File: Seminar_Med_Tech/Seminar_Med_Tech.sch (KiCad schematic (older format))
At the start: 25 parts

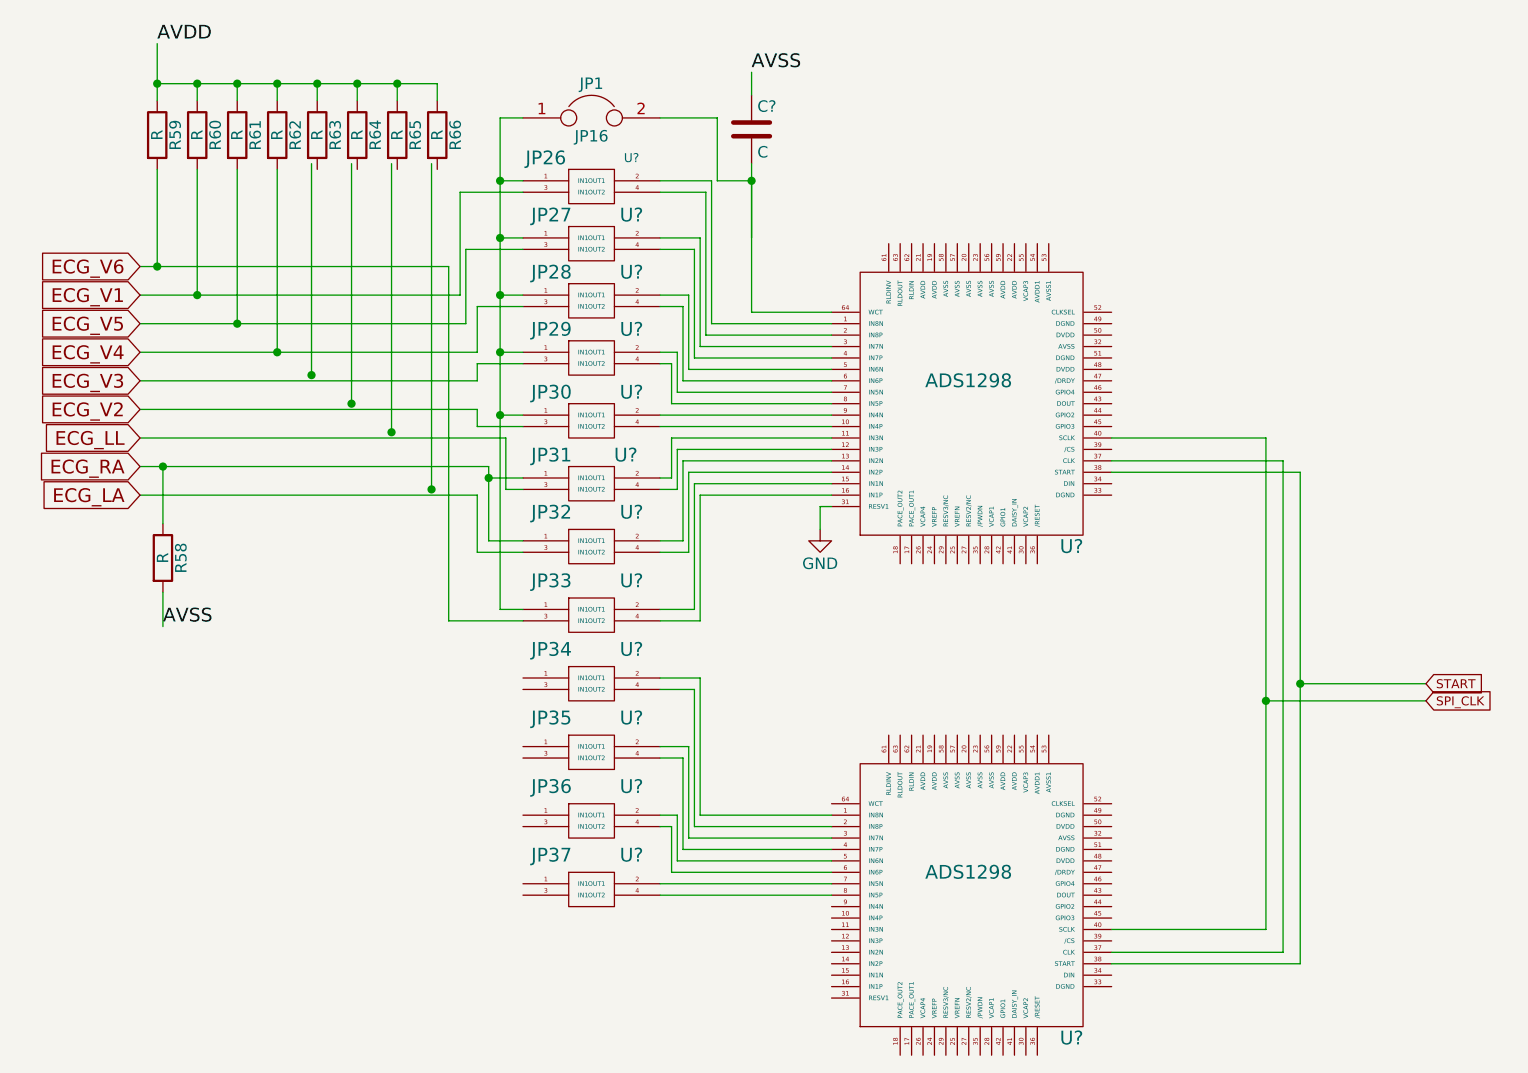
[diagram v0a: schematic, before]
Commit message: Tried to cascade the two chips
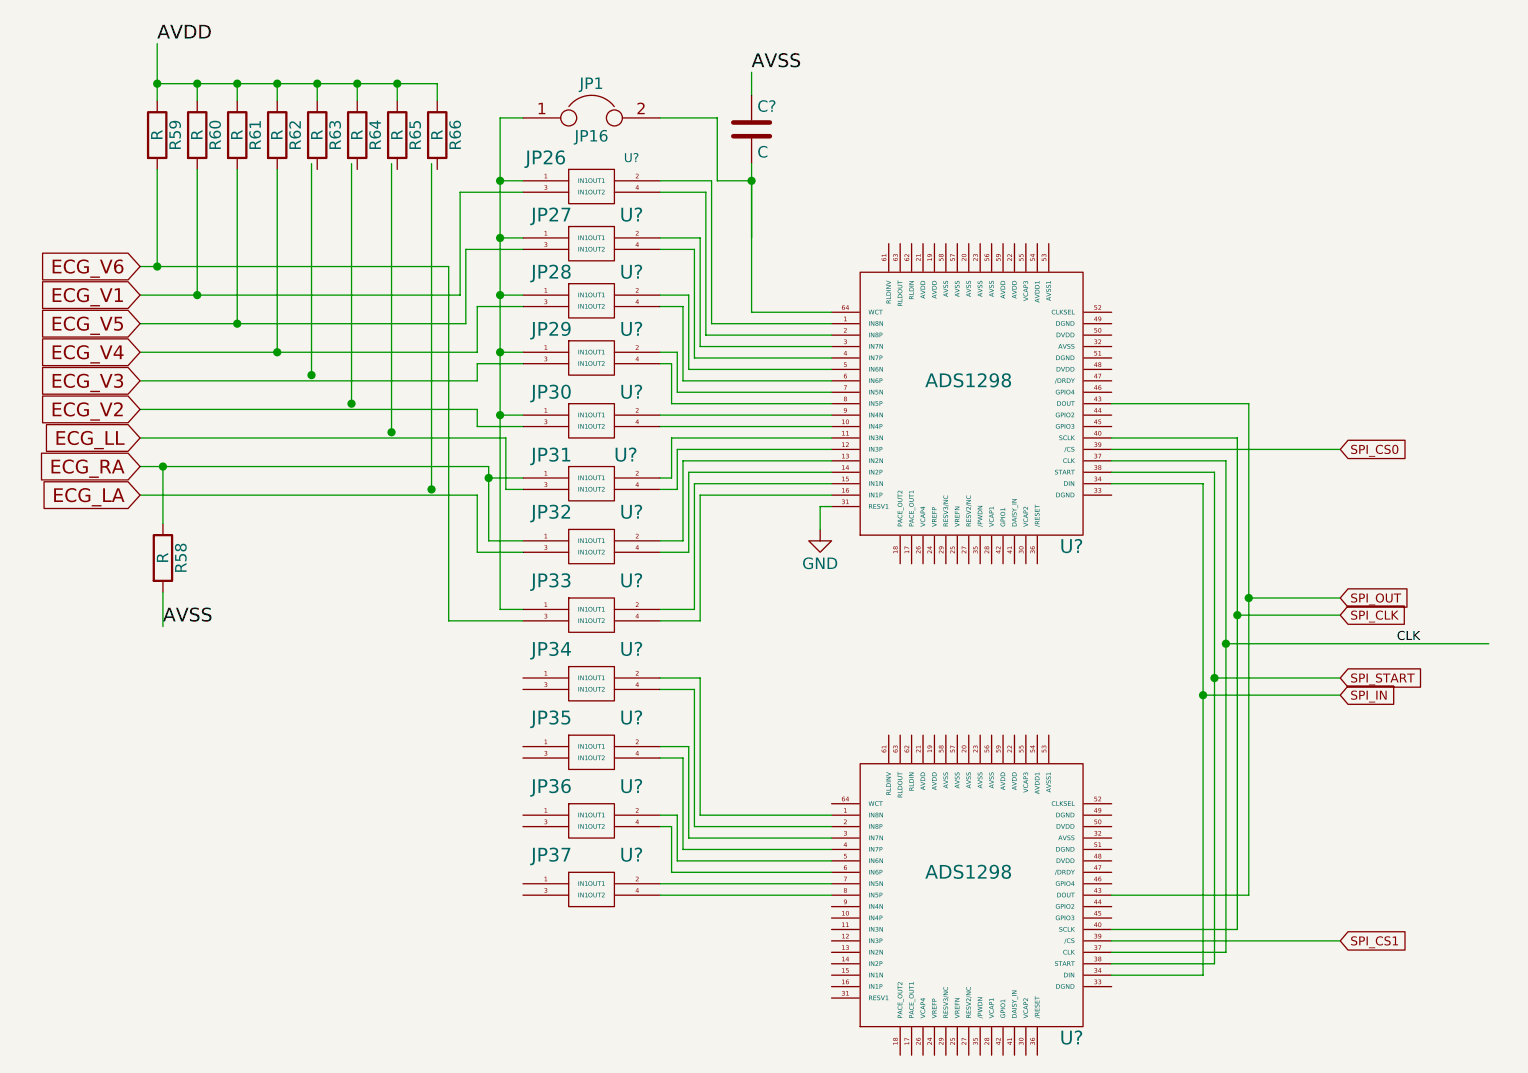
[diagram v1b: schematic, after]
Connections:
- net labels added: CLK, SPI_CS0, SPI_CS1, SPI_IN, SPI_OUT, SPI_START
- net labels removed: START
- wire segments 139 -> 150
